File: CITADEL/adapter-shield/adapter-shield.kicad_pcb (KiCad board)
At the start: 2 copper layers, 98 x 72 mm, 77 parts, among them J1 Angle Sensor, J10 Conn_01x02, J11 Conn_01x02, J12 Conn_01x02, J13 Conn_01x02, J14 Conn_01x04, J2 Conn_01x08, J3 Camera, J4 QWIIC_Generic_Conn, J5 USB_A, J6 Conn_01x02, J7 Conn_01x02, J8 Conn_01x02, J9 Conn_01x02, M1 Motor_Servo, M2 Motor_Servo, M3 Motor_Servo, M4 Motor_Servo, M5 Motor_Servo, Q1 Q_DUAL_PNP_PNP_C1B1B2C2E2E1, Q10 Q_PMOS_GSD, Q2 Q_NMOS_GSD, Q3 Q_NMOS_GSD, Q4 Q_NMOS_GSD, Q5 Q_NMOS_GSD, Q6 Q_NMOS_GSD, Q7 Q_NMOS_GSD, Q8 Q_NMOS_GSD, Q9 Q_NMOS_GSD, U1 AH1815-P-B, U10 LynxServo, U11 PCA9557, U2 AH1815-P-B, U3 3.3V LDO, U4 Pololu_Compact_TB67S249FTG, U5 Teensy_4.1, U6 AH1815-P-B, U7 AH1815-P-B, U8 TDK_I3A4W008A033V, U9 TDK_I3A4W008A033V

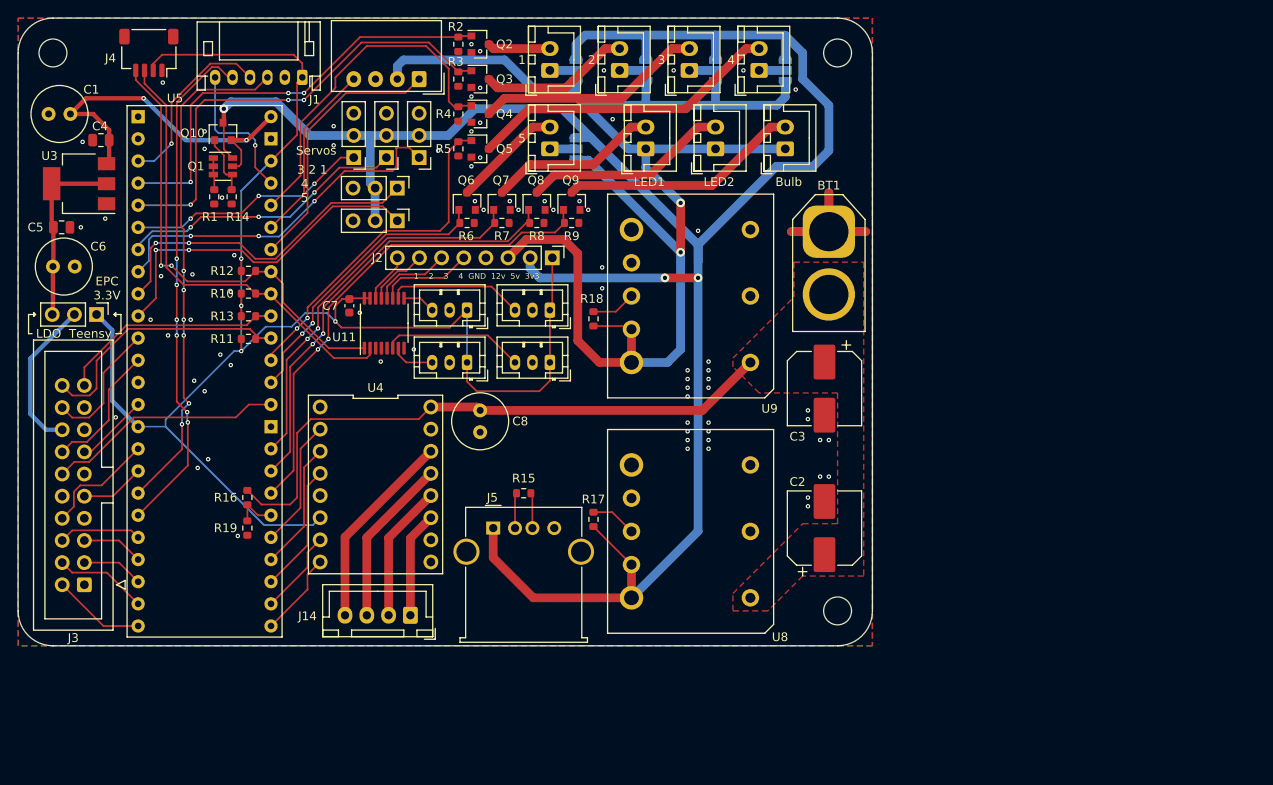
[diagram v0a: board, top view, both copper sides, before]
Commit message: CITADEL V2
April 14, 2022; Thomas Bennett
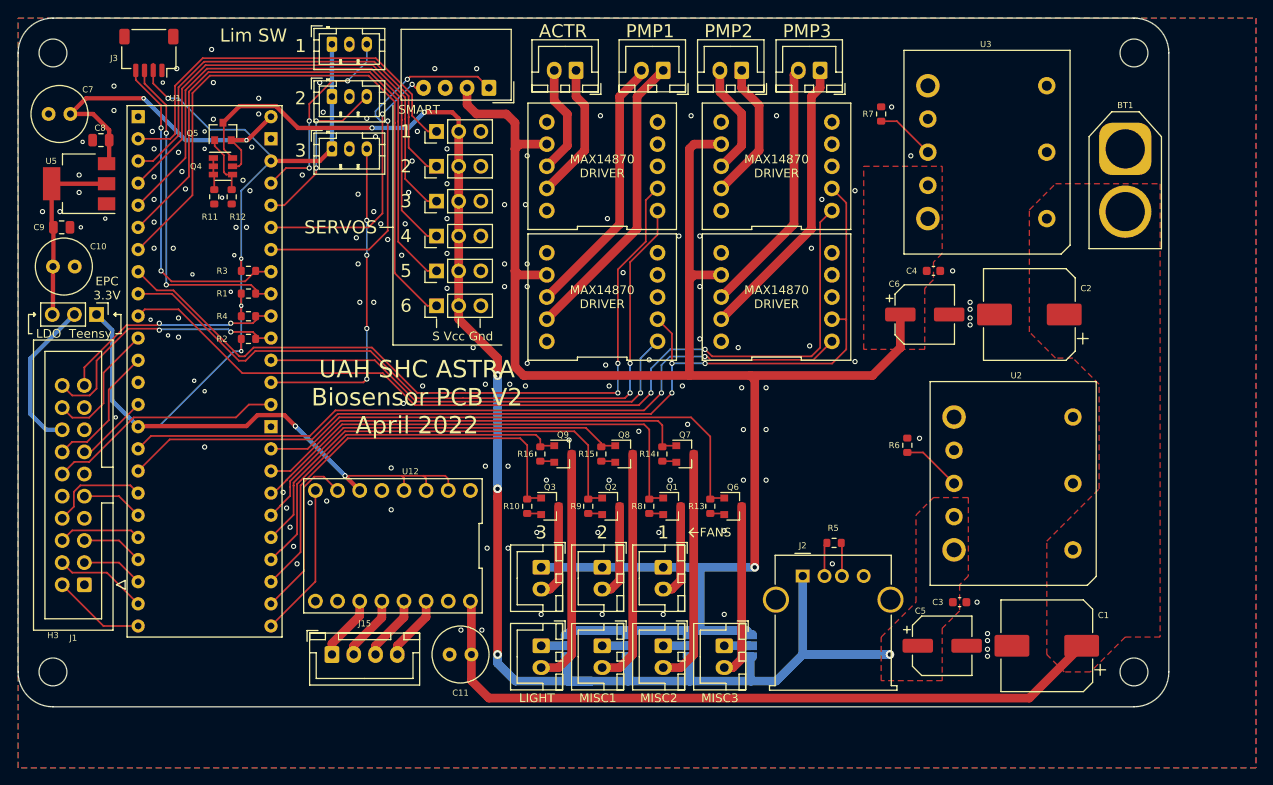
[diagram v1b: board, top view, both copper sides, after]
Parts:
- removed the C7 at (147.0, 139.4)
- removed the C8 at (162.0, 151.4)
- removed the J1 at (141.6, 113.2)
- removed the JP4 at (197.0, 112.4)
- removed the Q4 at (162.0, 117.4)
- removed the Q5 at (162.0, 121.4)
- removed R17: 8.45k, Resistor_SMD:R_0603_1608Metric
- removed R18: 1.82k, Resistor_SMD:R_0603_1608Metric
- removed R19: 10k, Resistor_SMD:R_0603_1608Metric
- removed the R2 at (159.5, 109.4)
- removed the R3 at (159.5, 113.4)
- removed the R4 at (159.5, 117.4)
- removed the U1 at (170.0, 145.9)
- added C1: 33u, Capacitor_SMD:CP_Elec_10x10, F.Cu at (227.0, 178.4)
- added C11: 100uF, Capacitor_THT:C_Radial_D6.3mm_H7.0mm_P2.50mm, F.Cu at (161.0, 179.4)
- added C4: 0.1u, Capacitor_SMD:C_0603_1608Metric, F.Cu at (214.0, 135.4)
- added C5: 22u, Capacitor_SMD:CP_Elec_6.3x5.9, F.Cu at (215.0, 178.4)
- added C6: 22u, Capacitor_SMD:CP_Elec_6.3x5.9, F.Cu at (213.0, 140.4)
- added H4: MountingHole, MountingHole:MountingHole_3.2mm_M3, F.Cu at (237.0, 181.4)
- added J15: Conn_01x04, Connector_JST:JST_XH_B4B-XH-A_1x04_P2.50mm_Vertical, F.Cu at (145.0, 179.4)
- added J4: Conn_01x02, Connector_JST:JST_XH_B2B-XH-A_1x02_P2.50mm_Vertical, F.Cu at (183.0, 169.4)
- added M6: Motor_Servo, Connector_PinHeader_2.54mm:PinHeader_1x03_P2.54mm_Vertical, F.Cu at (157.0, 139.4)
- added Q1: Q_NMOS_GSD, Package_TO_SOT_SMD:SOT-23, F.Cu at (184.0, 162.4)
- added R10: 10k, Resistor_SMD:R_0603_1608Metric, F.Cu at (167.4, 162.4)
- added R13: 10k, Resistor_SMD:R_0603_1608Metric, F.Cu at (188.4, 162.4)
- added R14: 10k, Resistor_SMD:R_0603_1608Metric, F.Cu at (182.9, 156.4)
- added U12: Pololu_Compact_TB67S249FTG, ASTRA_Footprints:DIP-16_500, F.Cu at (152.0, 166.9)
- added U13: AH1815-P-B, Connector_JST:JST_PH_B3B-PH-K_1x03_P2.00mm_Vertical, F.Cu at (145.0, 121.4)
- added U3: TDK_I3A4W008A033V, ASTRA_Footprints:Power_Supply_32nd_Brick, F.Cu at (227.0, 129.4)
- C2: footprint Capacitor_SMD:CP_Elec_8x5.4 -> Capacitor_SMD:CP_Elec_10x10
- C3: value 33u -> 0.1u; footprint Capacitor_SMD:CP_Elec_8x5.4 -> Capacitor_SMD:C_0603_1608Metric
- J14: value Conn_01x04 -> Conn_01x02; footprint Connector_JST:JST_XH_B4B-XH-A_1x04_P2.50mm_Vertical -> Connector_JST:JST_XH_B2B-XH-A_1x02_P2.50mm_Vertical
- J2: value Conn_01x08 -> USB_A; footprint Connector_PinHeader_2.54mm:PinHeader_1x08_P2.54mm_Vertical -> Connector_USB:USB_A_Molex_67643_Horizontal
- J5: value USB_A -> Conn_01x02; footprint Connector_USB:USB_A_Molex_67643_Horizontal -> Connector_JST:JST_XH_B2B-XH-A_1x02_P2.50mm_Vertical
- R15: value 200 -> 10k
- R16: value 113k -> 10k
- R5: value 10k -> 200
- R6: value 10k -> 8.45k
- R7: value 10k -> 1.82k
- U10: value LynxServo -> MAX14870_Breakout; footprint Connector_Molex:Molex_SPOX_5268-04A_1x04_P2.50mm_Horizontal -> ASTRA_Footprints:Pololu_2961
- U11: value PCA9557 -> MAX14870_Breakout; footprint Package_SO:TSSOP-16_4.4x5mm_P0.65mm -> ASTRA_Footprints:Pololu_2961
- U2: value AH1815-P-B -> TDK_I3A4W008A033V; footprint Connector_JST:JST_PH_B3B-PH-K_1x03_P2.00mm_Vertical -> ASTRA_Footprints:Power_Supply_32nd_Brick
- U4: value Pololu_Compact_TB67S249FTG -> LynxServo; footprint ASTRA_Footprints:DIP-16_500 -> Connector_Molex:Molex_SPOX_5268-04A_1x04_P2.50mm_Horizontal
- U8, U9: value TDK_I3A4W008A033V -> MAX14870_Breakout; footprint ASTRA_Footprints:Power_Supply_32nd_Brick -> ASTRA_Footprints:Pololu_2961
- moved H3 90.3 mm to (113.0, 181.4)
- moved J14 78.2 mm to (201.0, 112.4)
- moved U2 72.7 mm to (230.0, 167.4)
- moved JP1 69.0 mm to (193.0, 178.4), turned to 270 degrees
- moved J9 68.4 mm to (176.0, 178.4), turned to 270 degrees
- moved J7 67.1 mm to (190.0, 178.4), turned to 270 degrees
- moved JP3 66.8 mm to (179.0, 178.4), turned to 270 degrees
- moved JP2 66.2 mm to (186.0, 178.4), turned to 270 degrees
- moved J8 66.1 mm to (183.0, 178.4), turned to 270 degrees
- moved R5 62.5 mm to (202.6, 166.6), turned to 180 degrees
- moved J10 57.0 mm to (169.0, 178.4), turned to 270 degrees
- moved J6 57.0 mm to (169.0, 169.4), turned to 270 degrees
- moved JP5 57.0 mm to (172.0, 178.4), turned to 270 degrees
- moved R6 56.6 mm to (211.0, 155.4), turned to 90 degrees
- moved Q2 55.1 mm to (177.0, 162.4)
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- renumbered C6 to C10, C1 to C7, C4 to C8, C5 to C9, J3 to J1, J4 to J3, JP6 to JP4, Q1 to Q4, Q10 to Q5, R10 to R1, R1 to R11, R14 to R12, R11 to R2, R12 to R3, R13 to R4, U5 to U1, U3 to U5
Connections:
- C3 pad 1: /V_BAT -> +5VP
- J1 pad 10: /VDD_OA -> (no net)
- J1 pad 7: /GND_OA -> (no net)
- J11 pad 1: +12V -> Net-(J11-Pad1)
- J12 pad 1: +12V -> Net-(J12-Pad1)
- J13 pad 1: +12V -> Net-(J13-Pad1)
- J2 pad 1: +3V3 -> +5VP
- J2 pad 2: +5VP -> Net-(J2-Pad2)
- J2 pad 3: +12V -> Net-(J2-Pad3)
- J2 pad 5: /IO1 -> Net-(J2-Pad5)
- J5 pad 1: +5VP -> +12V
- J6 pad 1: Net-(J6-Pad1) -> +12V
- JP1 pad 2: Net-(J6-Pad1) -> Net-(J7-Pad1)
- JP2 pad 2: Net-(J7-Pad1) -> Net-(J8-Pad1)
- JP3 pad 2: Net-(J8-Pad1) -> Net-(J9-Pad1)
- Q2 pad 1: /MOSFET1 -> /FAN2
- Q2 pad 3: Net-(J6-Pad2) -> Net-(J5-Pad2)
- Q3 pad 1: /MOSFET2 -> /FAN3
- Q3 pad 3: Net-(J7-Pad2) -> Net-(J6-Pad2)
- Q6 pad 1: /MOSFET5 -> /LIGHT
- Q6 pad 3: Net-(J10-Pad2) -> Net-(J7-Pad2)
- Q7 pad 1: /LED1 -> /GEN1
- Q7 pad 3: Net-(J11-Pad2) -> Net-(J8-Pad2)
- Q8 pad 1: /LED2 -> /GEN2
- Q8 pad 3: Net-(J12-Pad2) -> Net-(J9-Pad2)
- Q9 pad 1: /BULB -> /GEN3
- Q9 pad 3: Net-(J13-Pad2) -> Net-(J10-Pad2)
- R15 pad 1: Net-(J5-Pad3) -> /GEN2
- R15 pad 2: Net-(J5-Pad2) -> GND
- R16 pad 1: /V_BAT -> /GEN3
- R16 pad 2: /V_BAT_Div -> GND
- R5 pad 1: /MOSFET4 -> Net-(J2-Pad3)
- R5 pad 2: GND -> Net-(J2-Pad2)
- R6 pad 1: /MOSFET5 -> Net-(R6-Pad1)
- R7 pad 1: /LED1 -> Net-(R7-Pad1)
- R8 pad 1: /LED2 -> /FAN1
- R9 pad 1: /BULB -> /FAN2
- U1 pad 10: /M5_PWM -> /Pump2_PWM
- U1 pad 13: Net-(U5-Pad13) -> (no net)
- U1 pad 18: /MOSFET5 -> /Hall_SW_3
- U1 pad 19: /MOSFET4 -> /Pump1_PWM
- U1 pad 2: Net-(U5-Pad2) -> /M1_PWM
- U1 pad 26: /MOSFET3 -> /Hall_SW_2
- U1 pad 27: /Angle_CS -> /Hall_SW_1
- U1 pad 3: /CIPO1 -> /M2_PWM
- U1 pad 31: /VIDEO_P -> /Pump3_PWM
- U1 pad 32: /VIDEO_N -> /Pump_DIR
- U1 pad 33: /COPI1 -> /VIDEO_P
- U1 pad 34: /SCK1 -> /VIDEO_N
- U1 pad 4: /MOSFET1 -> /M3_PWM
- U1 pad 42: /STEP_DMODE2 -> /FAN3
- U1 pad 43: /STEP_DMODE1 -> /GEN3
- U1 pad 44: /STEP_DMODE0 -> /FAN2
- U1 pad 45: /V_BAT_Div -> /GEN2
- U1 pad 46: /BULB -> /FAN1
- U1 pad 47: /LED2 -> /GEN1
- U1 pad 48: /LED1 -> /LIGHT
- U1 pad 5: /MOSFET2 -> /M4_PWM
- U1 pad 6: /M3_PWM -> /M5_PWM
- U1 pad 7: /M2_PWM -> /M6_PWM
- U1 pad 8: /M1_PWM -> /Act_DIR
- U1 pad 9: /M4_PWM -> /Act_PWM
- U10 pad 1: /Lynx_RX -> /Pump2_PWM
- U10 pad 2: +12V -> /Pump_DIR
- U10 pad 3: GND -> (no net)
- U10 pad 4: /Lynx_TX -> (no net)
- U11 pad 1: /QWIIC_SCL -> /Pump3_PWM
- U11 pad 10: /Hall_SW_4 -> (no net)
- U11 pad 2: /QWIIC_SDA -> /Pump_DIR
- U11 pad 3: GND -> (no net)
- U11 pad 4: GND -> (no net)
- U11 pad 6: /Hall_SW_1 -> GND
- U11 pad 7: /Hall_SW_2 -> +12V
- U11 pad 8: GND -> Net-(J14-Pad2)
- U11 pad 9: /Hall_SW_3 -> Net-(J14-Pad1)
- U2 pad 1: +3V3 -> /V_BAT
- U2 pad 2: GND -> (no net)
- U2 pad 3: /Hall_SW_2 -> GND
- U4 pad 1: Net-(U4-Pad1) -> /Lynx_RX
- U4 pad 2: /STEP_DMODE0 -> +12V
- U4 pad 3: /STEP_DMODE1 -> GND
- U4 pad 4: /STEP_DMODE2 -> /Lynx_TX
- U6 pad 3: /Hall_SW_3 -> /Hall_SW_1
- U7 pad 3: /Hall_SW_4 -> /Hall_SW_2
- U8 pad 1: /V_BAT -> /Act_PWM
- U8 pad 2: Net-(U8-Pad2) -> /Act_DIR
- U8 pad 3: GND -> (no net)
- U8 pad 4: GND -> (no net)
- U8 pad 5: Net-(U8-Pad5) -> GND
- U8 pad 6: Net-(R17-Pad2) -> GND
- U8 pad 7: +5VP -> +12V
- U8 pad 8: +5VP -> Net-(J11-Pad2)
- U9 pad 1: /V_BAT -> /Pump1_PWM
- U9 pad 2: Net-(U9-Pad2) -> /Pump_DIR
- U9 pad 3: GND -> (no net)
- U9 pad 4: GND -> (no net)
- U9 pad 5: Net-(U9-Pad5) -> GND
- U9 pad 6: Net-(R18-Pad2) -> GND
- U9 pad 8: +12V -> Net-(J12-Pad2)
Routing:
- net /Pump_DIR: track 0.00 -> 115.6 mm, vias 0 -> 3
- net /Pump2_PWM: track 0.00 -> 104.4 mm, vias 0 -> 2
- net /Act_DIR: track 0.00 -> 87.0 mm, vias 0 -> 2
- net /Pump3_PWM: track 0.00 -> 86.9 mm, vias 0 -> 2
- net /Act_PWM: track 0.00 -> 84.8 mm, vias 0 -> 2
- net +5VP: track 248.9 -> 168.8 mm, vias 3 -> 6
- net /M6_PWM: track 0.00 -> 71.8 mm
- net /LIGHT: track 0.00 -> 61.6 mm
- net /SCK1: track 58.8 -> 0.00 mm, vias 6 -> 0
- net /COPI1: track 58.4 -> 0.00 mm, vias 6 -> 0
- net /BULB: track 56.6 -> 0.00 mm, vias 2 -> 0
- net /FAN1: track 0.00 -> 56.6 mm
- net /MOSFET2: track 53.5 -> 0.00 mm, vias 3 -> 0
- net /Pump1_PWM: track 0.00 -> 52.2 mm, vias 0 -> 1
- net /FAN2: track 0.00 -> 52.1 mm
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- added copper zone on F.Cu, net +12V
- added copper zone on F.Cu, net +5VP
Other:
- board size 98 x 72 mm -> 132 x 79 mm
- board text added: "6"
- board text added: "ACTR"
- board text added: "FANS"
- board text added: "LIGHT"
- board text added: "Lim SW"
- board text added: "MAX14870 DRIVER"
- board text added: "MISC1"
- board text added: "MISC2"
- board text added: "MISC3"
- board text added: "PMP1"
- board text added: "PMP2"
- board text added: "PMP3"
- board text added: "S Vcc Gnd"
- board text added: "SERVOS"
- board text added: "SMART"
- board text added: "UAH SHC ASTRA Biosensor PCB V2 April 2022"
- board text removed: "1 2 3 4 GND 12v 5v 3v3"
- board text removed: "3 2 1 4 5"
- board text removed: "ASTRA Biosensor V1.5 Designed by Thomas Bennett 21 Sep 2021 Forked from Adrian Studer's EPC901 Adapter"
- board text removed: "Bulb"
- board text removed: "LED1"
- board text removed: "LED2"
- board text removed: "Servos"
